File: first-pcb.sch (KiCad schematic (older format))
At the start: 1 part

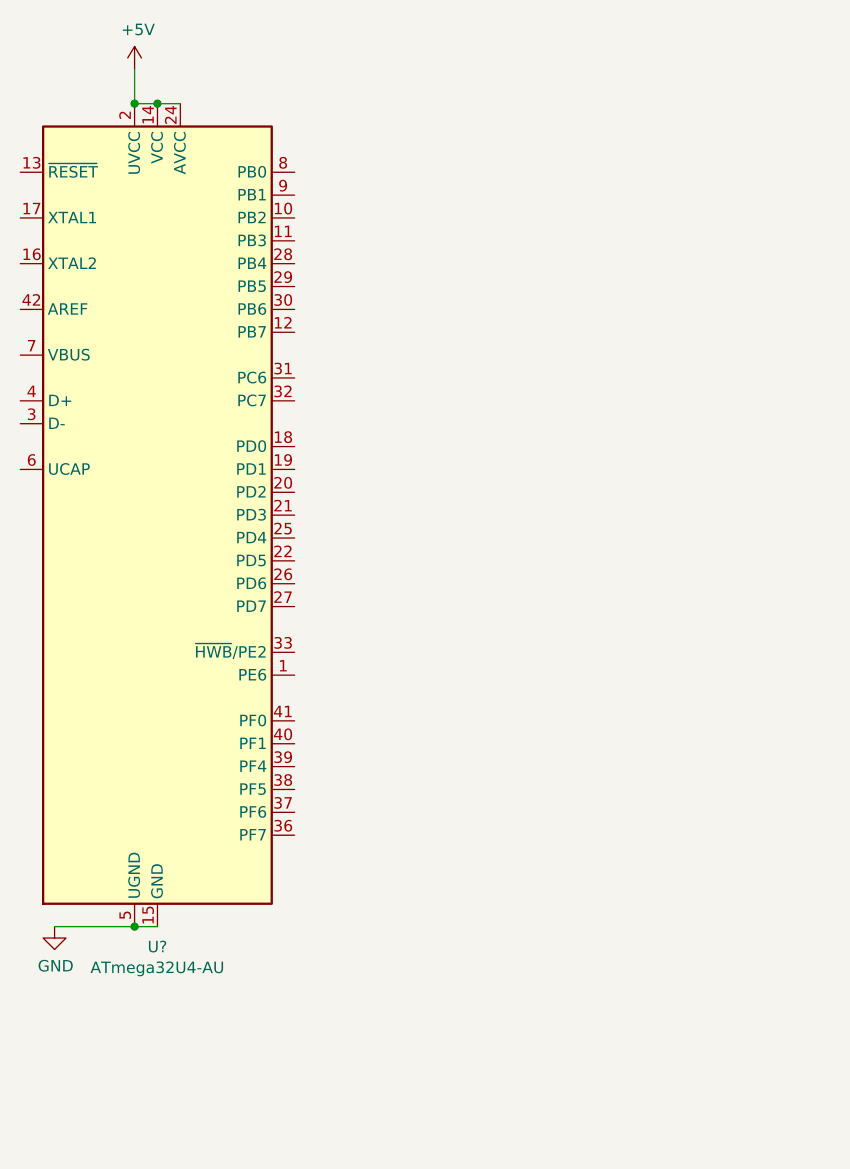
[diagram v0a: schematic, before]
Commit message: circut mcu started
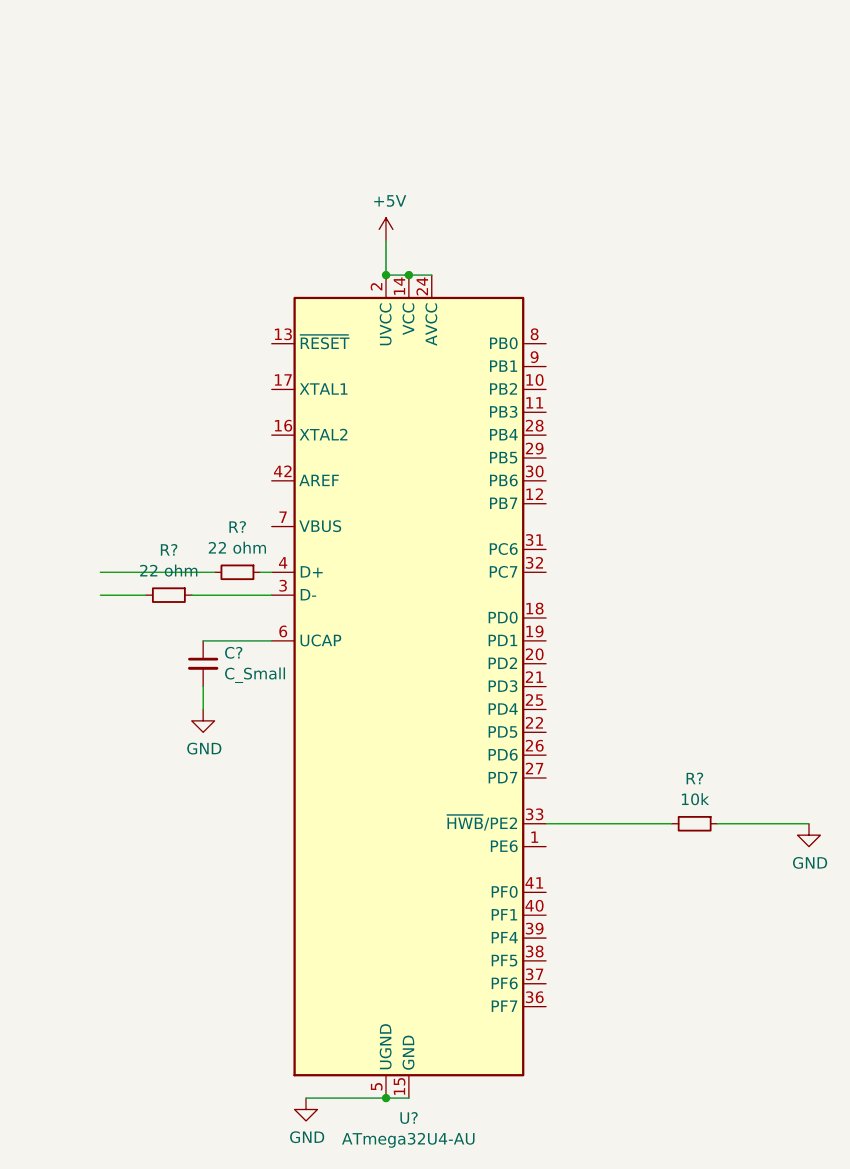
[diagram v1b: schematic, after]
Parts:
- added C?: C_Small, symbol Device:C_Small
- added R?: 10k, symbol Device:R_Small
- added R? (x2): 22 ohm, symbol Device:R_Small
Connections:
- wire segments 5 -> 13
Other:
- moved on the sheet: U?
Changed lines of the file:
@@
 $EndDescr
+$Comp
+L power:+5V #PWR?
+U 1 1 60890457
+P 2400 1550
+F 0 "#PWR?" H 2400 1400 50  0001 C CNN
+F 1 "+5V" H 2415 1723 50  0000 C CNN
+F 2 "" H 2400 1550 50  0001 C CNN
+F 3 "" H 2400 1550 50  0001 C CNN
+	1    2400 1550
+	1    0    0    -1
+$EndComp
+Wire Wire Line
+	2400 1700 2400 1550
+$Comp
+L power:GND #PWR?
+U 1 1 6089896B
+P 2050 5300
+F 0 "#PWR?" H 2050 5050 50  0001 C CNN
+F 1 "GND" H 2055 5127 50  0000 C CNN
+F 2 "" H 2050 5300 50  0001 C CNN
+F 3 "" H 2050 5300 50  0001 C CNN
+	1    2050 5300
+	1    0    0    -1
+$EndComp
+$Comp
+L power:GND #PWR?
+U 1 1 608B4E9F
+P 4250 4100
+F 0 "#PWR?" H 4250 3850 50  0001 C CNN
+F 1 "GND" H 4255 3927 50  0000 C CNN
+F 2 "" H 4250 4100 50  0001 C CNN
+F 3 "" H 4250 4100 50  0001 C CNN
+	1    4250 4100
+	1    0    0    -1
+$EndComp
+$Comp
+L Device:R_Small R?
+U 1 1 608B3B9E
+P 3750 4100
+F 0 "R?" V 3554 4100 50  0000 C CNN
+F 1 "10k" V 3645 4100 50  0000 C CNN
+F 2 "" H 3750 4100 50  0001 C CNN
+F 3 "~" H 3750 4100 50  0001 C CNN
+	1    3750 4100
+	0    1    1    0
+$EndComp
+Wire Wire Line
+	3850 4100 4250 4100
+$Comp
+L Device:R_Small R?
+U 1 1 608C1A01
+P 1450 3100
+F 0 "R?" V 1254 3100 50  0000 C CNN
+F 1 "22 ohm" V 1345 3100 50  0000 C CNN
+F 2 "" H 1450 3100 50  0001 C CNN
+F 3 "~" H 1450 3100 50  0001 C CNN
+	1    1450 3100
+	0    1    1    0
+$EndComp
+$Comp
+L Device:R_Small R?
+U 1 1 608C25D5
+P 1750 3000
+F 0 "R?" V 1554 3000 50  0000 C CNN
+F 1 "22 ohm" V 1645 3000 50  0000 C CNN
+F 2 "" H 1750 3000 50  0001 C CNN
+F 3 "~" H 1750 3000 50  0001 C CNN
+	1    1750 3000
+	0    1    1    0
+$EndComp
+Wire Wire Line
+	2400 1700 2500 1700
+Wire Wire Line
+	2500 1700 2600 1700
+Connection ~ 2400 1700
+Connection ~ 2500 1700
+Connection ~ 2400 5300
+Wire Wire Line
+	2050 5300 2400 5300
+Wire Wire Line
+	2400 5300 2500 5300
+Wire Wire Line
+	3100 4100 3650 4100
 $Comp
 L MCU_Microchip_ATmega:ATmega32U4-AU U?
 U 1 1 608618EE
-P 1400 2750
-F 0 "U?" H 1400 861 50  0000 C CNN
-F 1 "ATmega32U4-AU" H 1400 770 50  0000 C CNN
-F 2 "Package_QFP:TQFP-44_10x10mm_P0.8mm" H 1400 2750 50  0001 C CIN
-F 3 "http://ww1.microchip.com/downloads/en/DeviceDoc/Atmel-7766-8-bit-AVR-ATmega16U4-32U4_Datasheet.pdf" H 1400 2750 50  0001 C CNN
-	1    1400 2750
-	1    0    0    -1
-$EndComp
-$Comp
-L power:+5V #PWR?
-U 1 1 60890457
-P 1300 800
-F 0 "#PWR?" H 1300 650 50  0001 C CNN
-F 1 "+5V" H 1315 973 50  0000 C CNN
-F 2 "" H 1300 800 50  0001 C CNN
-F 3 "" H 1300 800 50  0001 C CNN
-	1    1300 800
+P 2500 3500
+F 0 "U?" H 2500 1611 50  0000 C CNN
+F 1 "ATmega32U4-AU" H 2500 1520 50  0000 C CNN
+F 2 "Package_QFP:TQFP-44_10x10mm_P0.8mm" H 2500 3500 50  0001 C CIN
+F 3 "http://ww1.microchip.com/downloads/en/DeviceDoc/Atmel-7766-8-bit-AVR-ATmega16U4-32U4_Datasheet.pdf" H 2500 3500 50  0001 C CNN
+	1    2500 3500
 	1    0    0    -1
 $EndComp
 Wire Wire Line
-	1300 950  1300 800
+	1900 3000 1850 3000
 Wire Wire Line
-	1300 950  1400 950
-Connection ~ 1300 950
-Connection ~ 1400 950
+	1150 3000 1650 3000
 Wire Wire Line
-	1400 950  1500 950
+	1900 3100 1550 3100
+Wire Wire Line
+	1150 3100 1350 3100
 $Comp
-L power:GND #PWR?
-U 1 1 6089896B
-P 950 4550
-F 0 "#PWR?" H 950 4300 50  0001 C CNN
-F 1 "GND" H 955 4377 50  0000 C CNN
-F 2 "" H 950 4550 50  0001 C CNN
-F 3 "" H 950 4550 50  0001 C CNN
-	1    950  4550
+L Device:C_Small C?
+U 1 1 608D8F91
+P 1600 3400
+F 0 "C?" H 1692 3446 50  0000 L CNN
+F 1 "C_Small" H 1692 3355 50  0000 L CNN
+F 2 "" H 1600 3400 50  0001 C CNN
+F 3 "~" H 1600 3400 50  0001 C CNN
+	1    1600 3400
 	1    0    0    -1
 $EndComp
 Wire Wire Line
-	950  4550 1300 4550
-Connection ~ 1300 4550
+	1600 3300 1900 3300
+$Comp
+L power:GND #PWR?
+U 1 1 608DB4F9
+P 1600 3600
+F 0 "#PWR?" H 1600 3350 50  0001 C CNN
+F 1 "GND" H 1605 3427 50  0000 C CNN
+F 2 "" H 1600 3600 50  0001 C CNN
+F 3 "" H 1600 3600 50  0001 C CNN
+	1    1600 3600
+	1    0    0    -1
+$EndComp
 Wire Wire Line
-	1300 4550 1400 4550
+	1600 3500 1600 3600
 $EndSCHEMATC
